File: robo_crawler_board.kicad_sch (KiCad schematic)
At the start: 30 parts, among them J1 Screw_Terminal_01x02, J2 Screw_Terminal_01x02, J3 Screw_Terminal_01x02, J4 Screw_Terminal_01x02, J5 Screw_Terminal_01x02, J6 Screw_Terminal_01x02, J7 Screw_Terminal_01x02, J8 Screw_Terminal_01x02, J9 Screw_Terminal_01x02, Q1 IRLZ44N, Q2 IRLZ44N, U1 DRV8871DDA, U2 DRV8871DDA, U3 DRV8871DDA, U4 DRV8871DDA, U8 DRV8871DDA, U9 DRV8871DDA

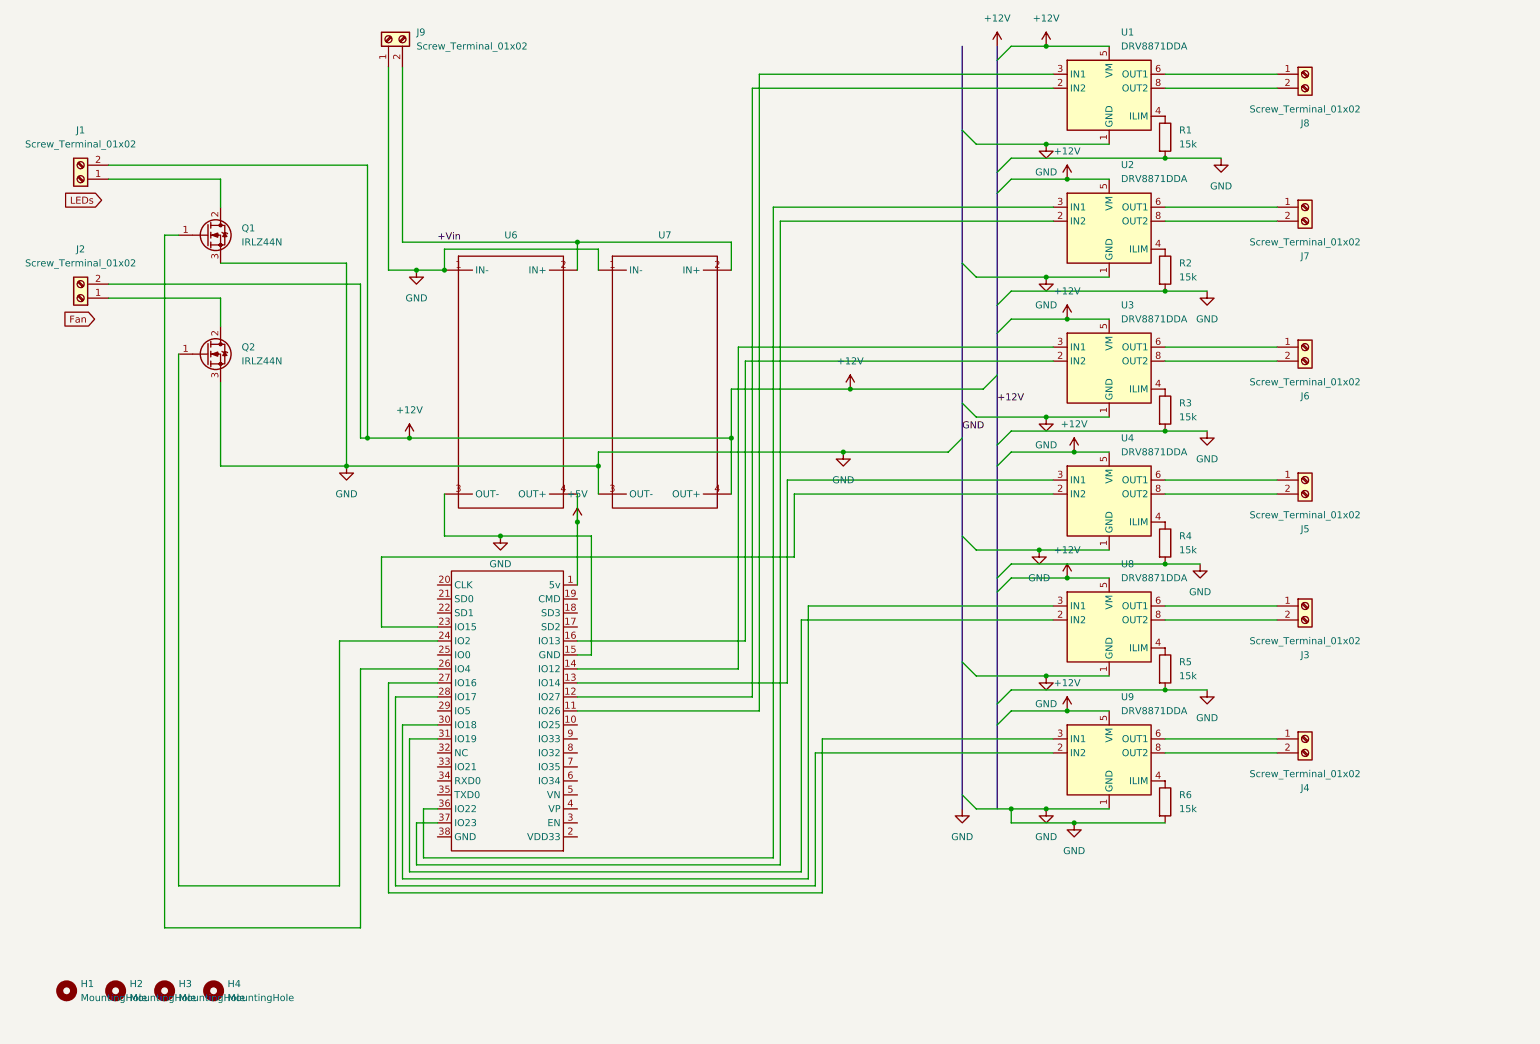
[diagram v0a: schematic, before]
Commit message: Reworking board design
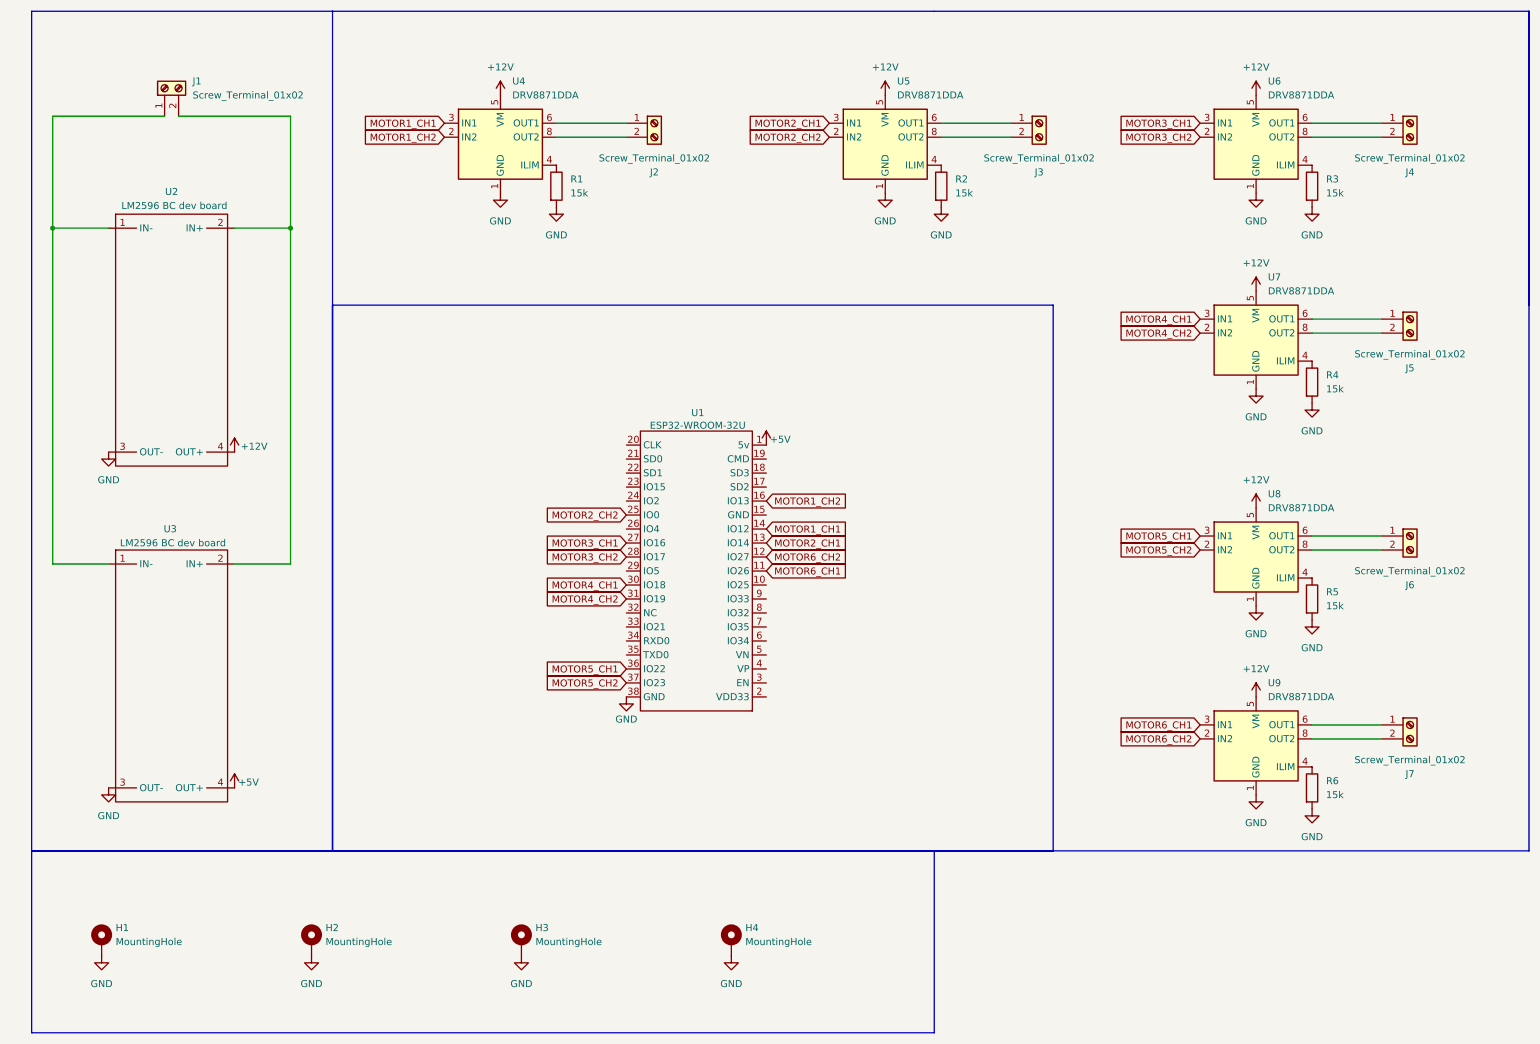
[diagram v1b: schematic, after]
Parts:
- removed J1, J2: Screw_Terminal_01x02, TerminalBlock:TerminalBlock_bornier-2_P5.08mm, symbol Connector:Screw_Terminal_01x02
- removed Q1, Q2: IRLZ44N, Package_TO_SOT_THT:TO-220-3_Vertical, symbol Transistor_FET:IRLZ44N
- removed U2, U3, U4: DRV8871DDA, Package_SO:Texas_HTSOP-8-1EP_3.9x4.9mm_P1.27mm_EP2.95x4.9mm_Mask2.4x3.1mm_ThermalVias, symbol Driver_Motor:DRV8871DDA
- added U5, U6, U7: DRV8871DDA, Package_SO:Texas_HTSOP-8-1EP_3.9x4.9mm_P1.27mm_EP2.95x4.9mm_Mask2.4x3.1mm_ThermalVias, symbol Driver_Motor:DRV8871DDA
- H1, H2, H3, H4: footprint MountingHole:MountingHole_2.2mm_M2 -> MountingHole:MountingHole_2.2mm_M2_Pad; symbol Mechanical:MountingHole -> Mechanical:MountingHole_Pad
- U2: renamed from U6; Part Name (none) -> LM2596 BC dev board
- renumbered J9 to J1, J8 to J2, U5 to U1, U7 to U3, U1 to U4
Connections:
- net +12V: now also U2.4 (OUT+), U5.5 (VM), U6.5 (VM), U7.5 (VM); no longer U3.4 (OUT+)
- net +5V: now also U3.4 (OUT+); no longer U2.4 (OUT+)
- net GND: now also H1.1, H2.1, H3.1, H4.1, U1.38 (GND), U5.1 (GND), U5.7 (GND), U5.9 (GND), U6.1 (GND), U6.7 (GND), U6.9 (GND), U7.1 (GND), U7.7 (GND), U7.9 (GND); no longer J1.1 (Pin_1), U1.15 (GND), U2.1 (IN-), U3.1 (IN-)
- net MOTOR1_CH2: now reaches U4.2 (IN2)
- net MOTOR1_CH2: now also U1.16 (IO13); no longer U1.12 (IO27)
- net MOTOR1_CH1: now reaches U4.3 (IN1)
- net MOTOR1_CH1: now also U1.14 (IO12); no longer U1.11 (IO26)
- net at J5.1 (Pin_1): now also U7.6 (OUT1)
- net at J5.2 (Pin_2): now also U7.8 (OUT2)
- net at J7.1 (Pin_1): now also U9.6 (OUT1)
- net at J7.2 (Pin_2): now also U9.8 (OUT2)
- net MOTOR5_CH2: now reaches U1.37 (IO23)
- net MOTOR5_CH2: now also U8.2 (IN2)
- net MOTOR5_CH1: now reaches U1.36 (IO22)
- net MOTOR5_CH1: now also U8.3 (IN1)
- net at R2.1: now also U5.4 (ILIM)
- net MOTOR2_CH1: now reaches U1.13 (IO14)
- net MOTOR2_CH1: now also U5.3 (IN1)
- net MOTOR2_CH2: now reaches U1.25 (IO0)
- net MOTOR2_CH2: now also U5.2 (IN2)
- net MOTOR3_CH1: now reaches U1.27 (IO16)
- net MOTOR3_CH1: now also U6.3 (IN1); no longer U9.3 (IN1)
- net MOTOR3_CH2: now reaches U1.28 (IO17)
- net MOTOR3_CH2: now also U6.2 (IN2); no longer U9.2 (IN2)
- net MOTOR4_CH1: now reaches U1.30 (IO18)
- net MOTOR4_CH1: now also U7.3 (IN1); no longer U8.3 (IN1)
- net MOTOR4_CH2: now reaches U1.31 (IO19)
- net MOTOR4_CH2: now also U7.2 (IN2); no longer U8.2 (IN2)
- net at R4.1: now also U7.4 (ILIM)
- net at J4.1 (Pin_1): now also U6.6 (OUT1); no longer U9.6 (OUT1)
- net at J4.2 (Pin_2): now also U6.8 (OUT2); no longer U9.8 (OUT2)
- net at U8.6 (OUT1): now also J6.1 (Pin_1); no longer J3.1 (Pin_1)
- net at U8.8 (OUT2): now also J6.2 (Pin_2); no longer J3.2 (Pin_2)
- net at R3.1: now also U6.4 (ILIM)
- net +Vin: no longer names the net of J1.2 (Pin_2), U2.2 (IN+), U3.2 (IN+)
- new net: J1.1 (Pin_1), U2.1 (IN-), U3.1 (IN-)
- new net: J3.1 (Pin_1), U5.6 (OUT1)
- new net: J3.2 (Pin_2), U5.8 (OUT2)
- new net MOTOR6_CH1: U1.11 (IO26), U9.3 (IN1)
- new net MOTOR6_CH2: U1.12 (IO27), U9.2 (IN2)
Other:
- moved on the sheet: J1, J2, R1, U2, U3, U4
